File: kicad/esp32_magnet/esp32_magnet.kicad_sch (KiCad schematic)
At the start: 26 parts, among them J1 USB_C_Receptacle_USB2.0_16P, J3 OV5640_LED, U1 ESP32-S3-WROOM-1, U2 AMS1117

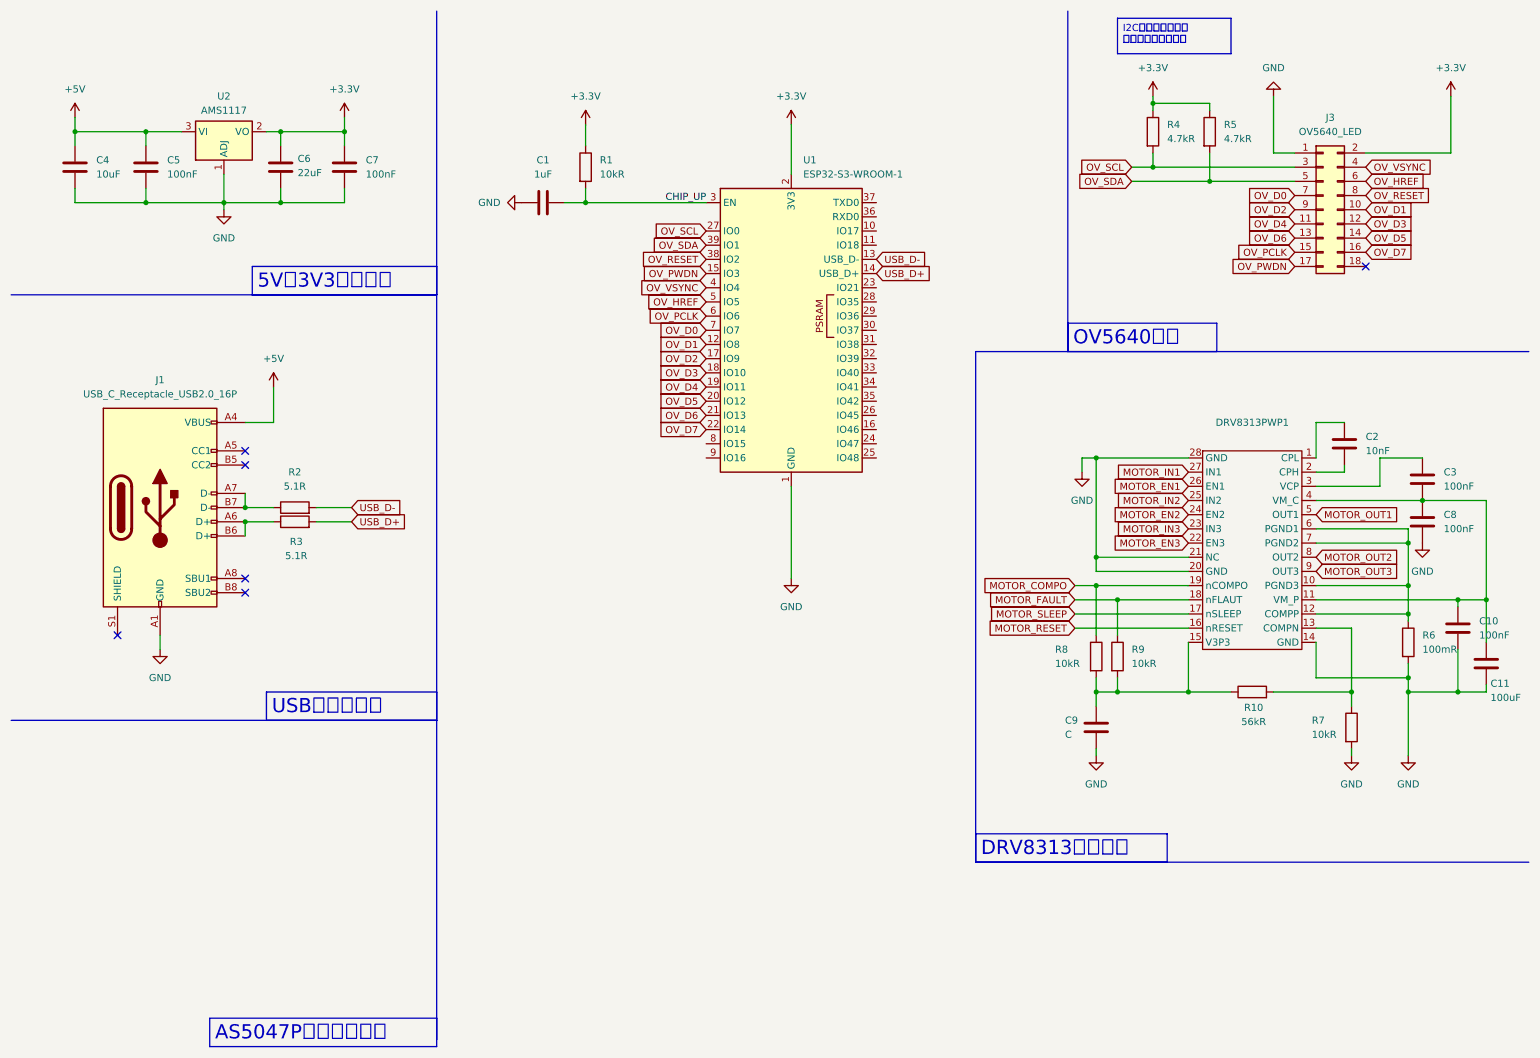
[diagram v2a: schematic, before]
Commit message: fix(kicad):as5047p
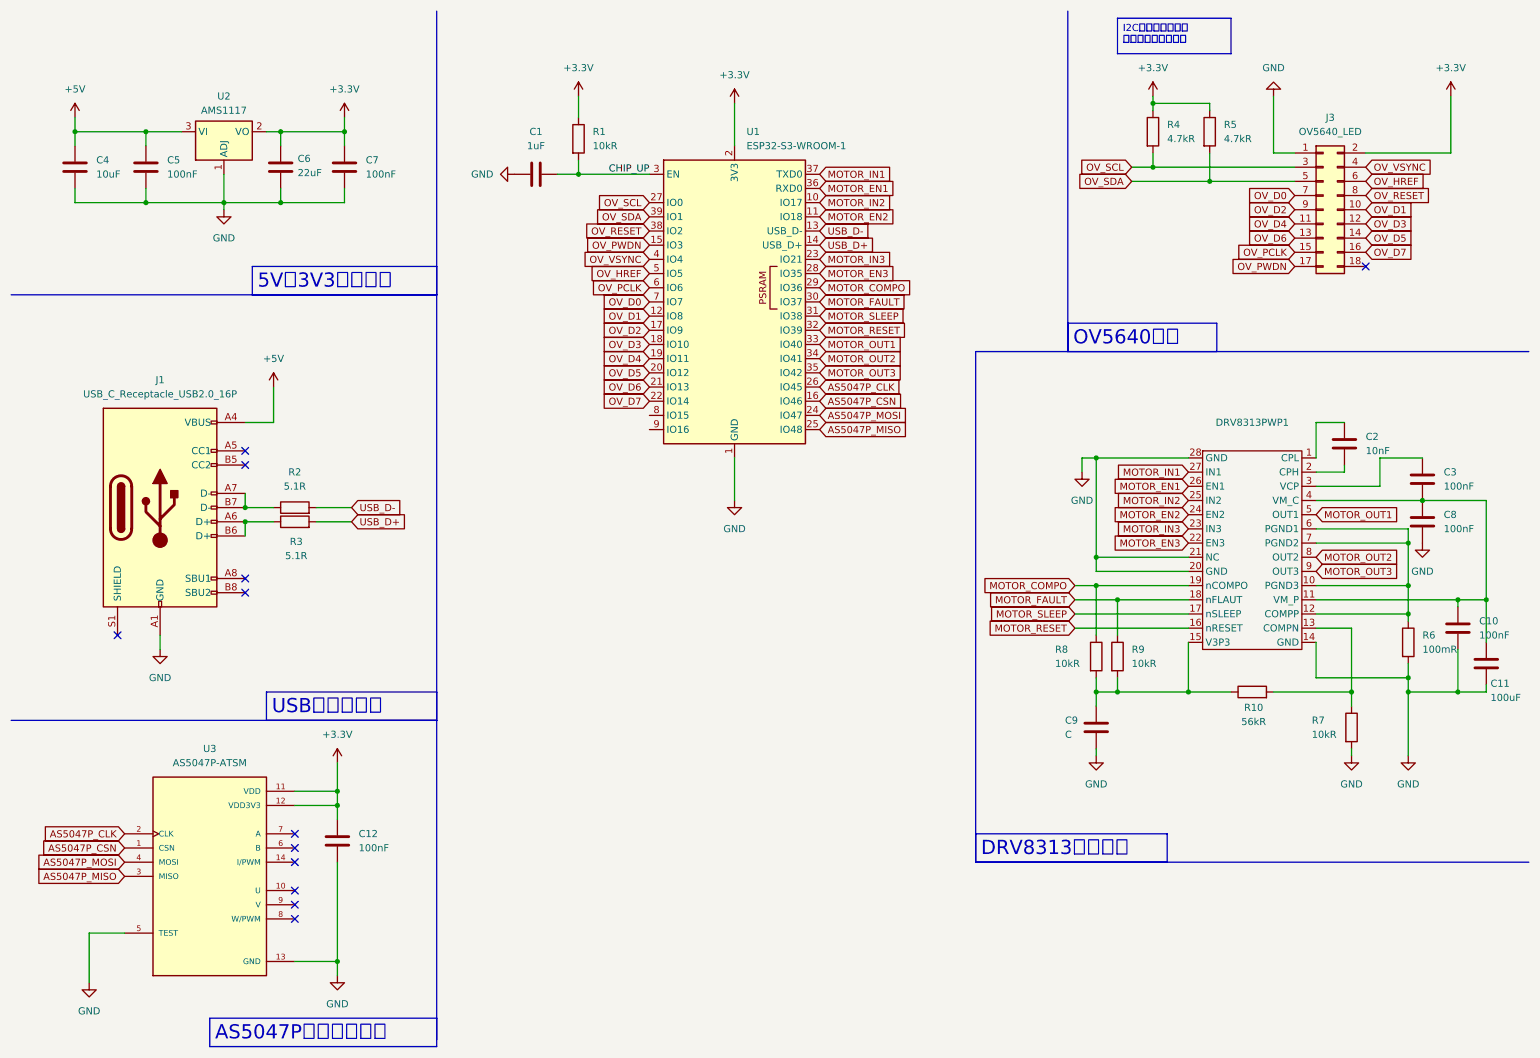
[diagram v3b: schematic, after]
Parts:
- added C12: 100nF, Capacitor_SMD:C_0603_1608Metric, symbol Device:C
- added U3: AS5047P-ATSM, Driver_IC:AS5047P-ATSM, symbol Driver_IC:AS5047P-ATSM
- DRV8313PWP1: footprint DriverIC:DRV8313PWP-SOP65P640X120-29N -> Driver_IC:SOP65P640X120-29N
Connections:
- net +3.3V: now also C12.1, U3.11 (VDD), U3.12 (VDD3V3)
- net GND: now also C12.2, U3.13 (GND), U3.5 (TEST)
- net MOTOR_COMPO: now also U1.29 (IO36)
- net MOTOR_EN1: now also U1.36 (RXD0)
- net MOTOR_EN2: now also U1.11 (IO18)
- net MOTOR_EN3: now also U1.28 (IO35)
- net MOTOR_FAULT: now also U1.30 (IO37)
- net MOTOR_IN1: now also U1.37 (TXD0)
- net MOTOR_IN2: now also U1.10 (IO17)
- net MOTOR_IN3: now also U1.23 (IO21)
- net MOTOR_OUT1: now also U1.33 (IO40)
- net MOTOR_OUT2: now also U1.34 (IO41)
- net MOTOR_OUT3: now also U1.35 (IO42)
- net MOTOR_RESET: now also U1.32 (IO39)
- net MOTOR_SLEEP: now also U1.31 (IO38)
- net AS5047P_CSN: now reaches U1.16 (IO46)
- net AS5047P_CSN: now also U3.1 (CSN)
- net AS5047P_MOSI: now reaches U1.24 (IO47)
- net AS5047P_MOSI: now also U3.4 (MOSI)
- net AS5047P_MISO: now reaches U1.25 (IO48)
- net AS5047P_MISO: now also U3.3 (MISO)
- net AS5047P_CLK: now reaches U1.26 (IO45)
- net AS5047P_CLK: now also U3.2 (CLK)
- no-connect marks 6 -> 12
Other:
- moved on the sheet: C1, R1, U1

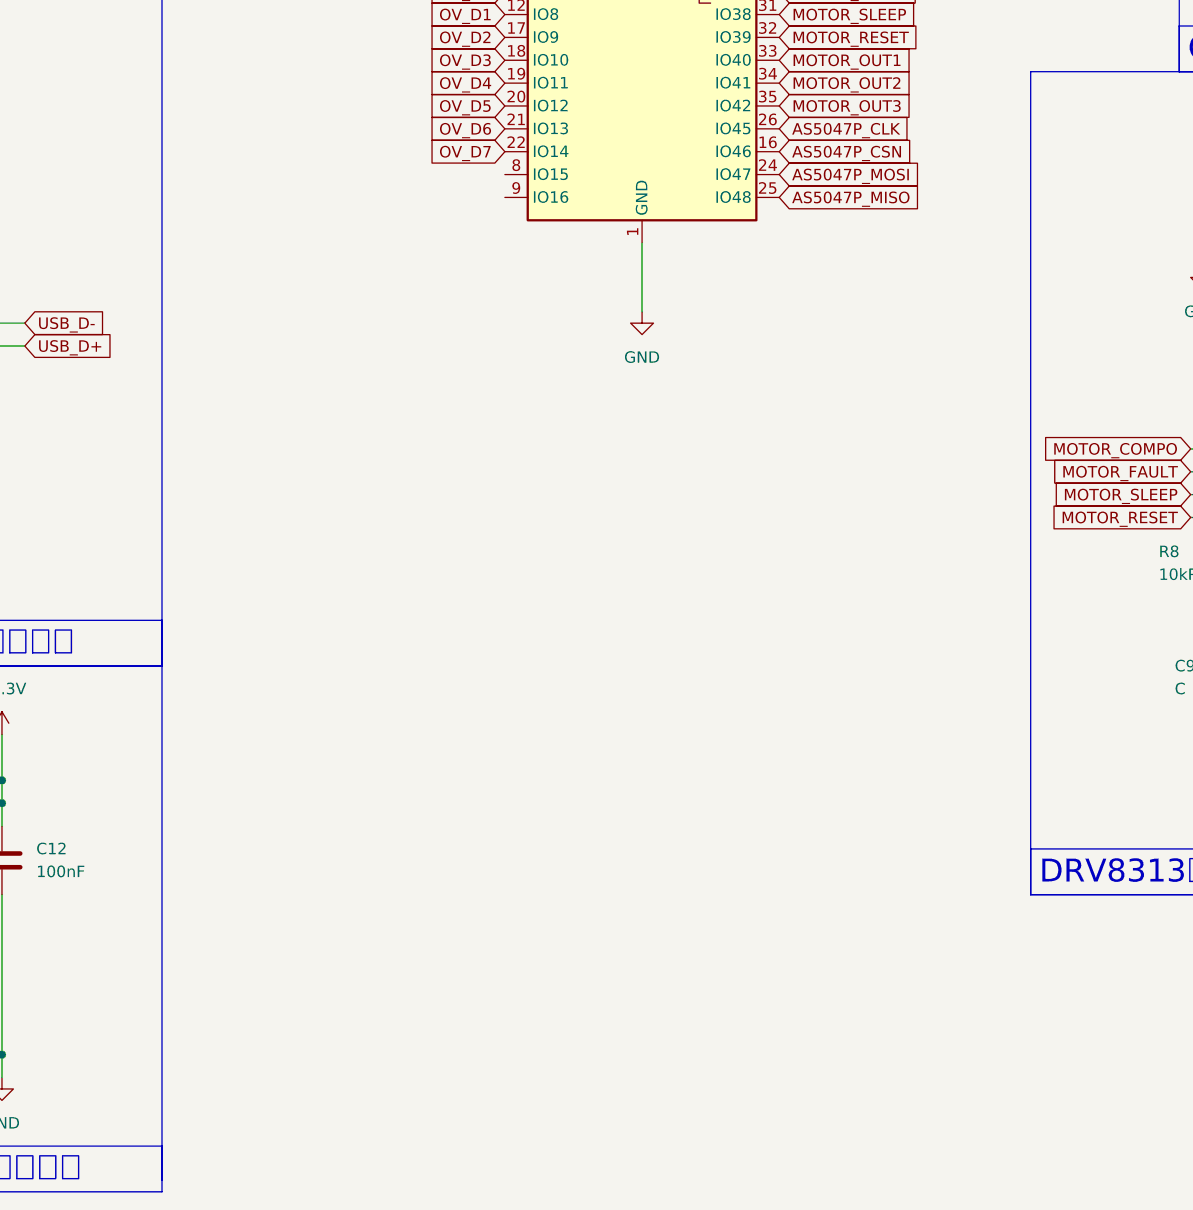
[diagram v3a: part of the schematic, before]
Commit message: fix(kicad):dy-sv17f
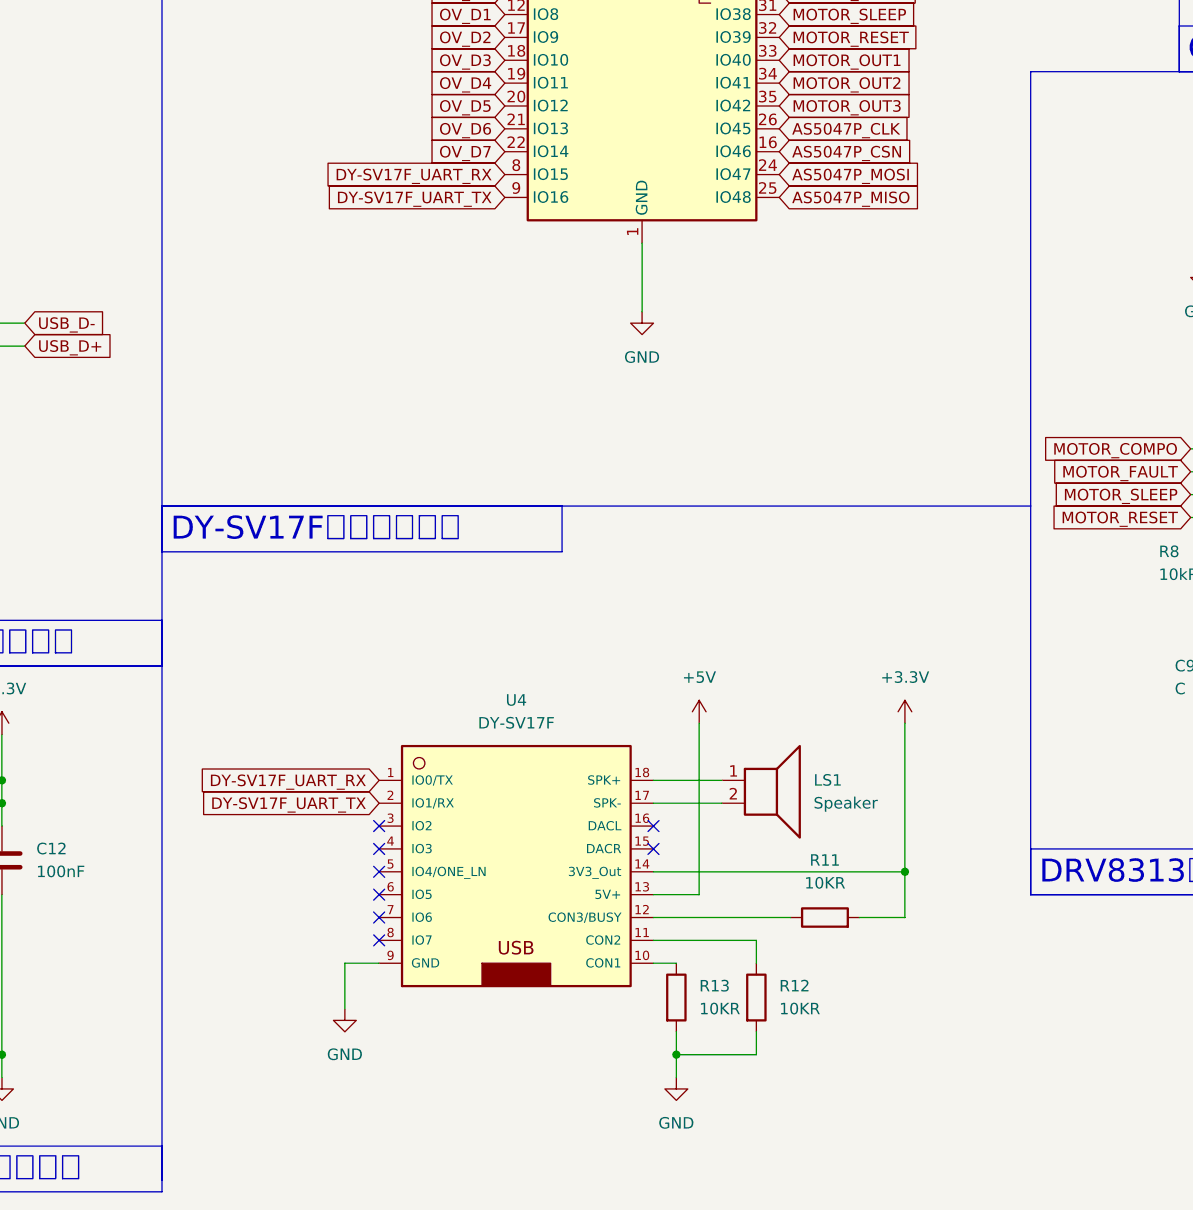
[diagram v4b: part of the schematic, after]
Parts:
- added LS1: Speaker, symbol Device:Speaker
- added R11, R12, R13: 10KR, Resistor_SMD:R_1206_3216Metric, symbol Device:R
- added U4: DY-SV17F, Audio_Driver_IC:DY-SV17F, symbol Audio_Driver_IC:DY-SV17F
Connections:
- net +3.3V: now also R11.2, U4.14 (3V3_Out)
- net +5V: now also U4.13 (5V+)
- net GND: now also R12.2, R13.2, U4.9 (GND)
- net DY-SV17F_UART_RX: now reaches U1.8 (IO15)
- net DY-SV17F_UART_RX: now also U4.1 (IO0/TX)
- net DY-SV17F_UART_TX: now reaches U1.9 (IO16)
- net DY-SV17F_UART_TX: now also U4.2 (IO1/RX)
- new net: R12.1, U4.11 (CON2)
- new net: LS1.1, U4.18 (SPK+)
- new net: LS1.2, U4.17 (SPK-)
- new net: R13.1, U4.10 (CON1)
- new net: R11.1, U4.12 (CON3/BUSY)
- no-connect marks 12 -> 20
